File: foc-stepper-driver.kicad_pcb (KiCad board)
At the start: 4 copper layers, 42 x 42 mm, 72 parts, among them CN1 C42391660, CN2 C2839706, CN3 C2839705, CN4 C2839704, J2 TC2030, U1 DRV8962DDWR, U2 TYPE-C 16PLT-H10.0, U3 STM32G431CBT6, U6 AS5047P-ATSM, U7 TPS560430XDBVR, U8 SPX3819M5-L-3-3/TR, U9 TCAN3403DRQ1, X1 NX3215SA 32.768KHZ EXS00A-MU0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, X2 NDK NX2016SA-24MHZ-EXS00A-CS1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

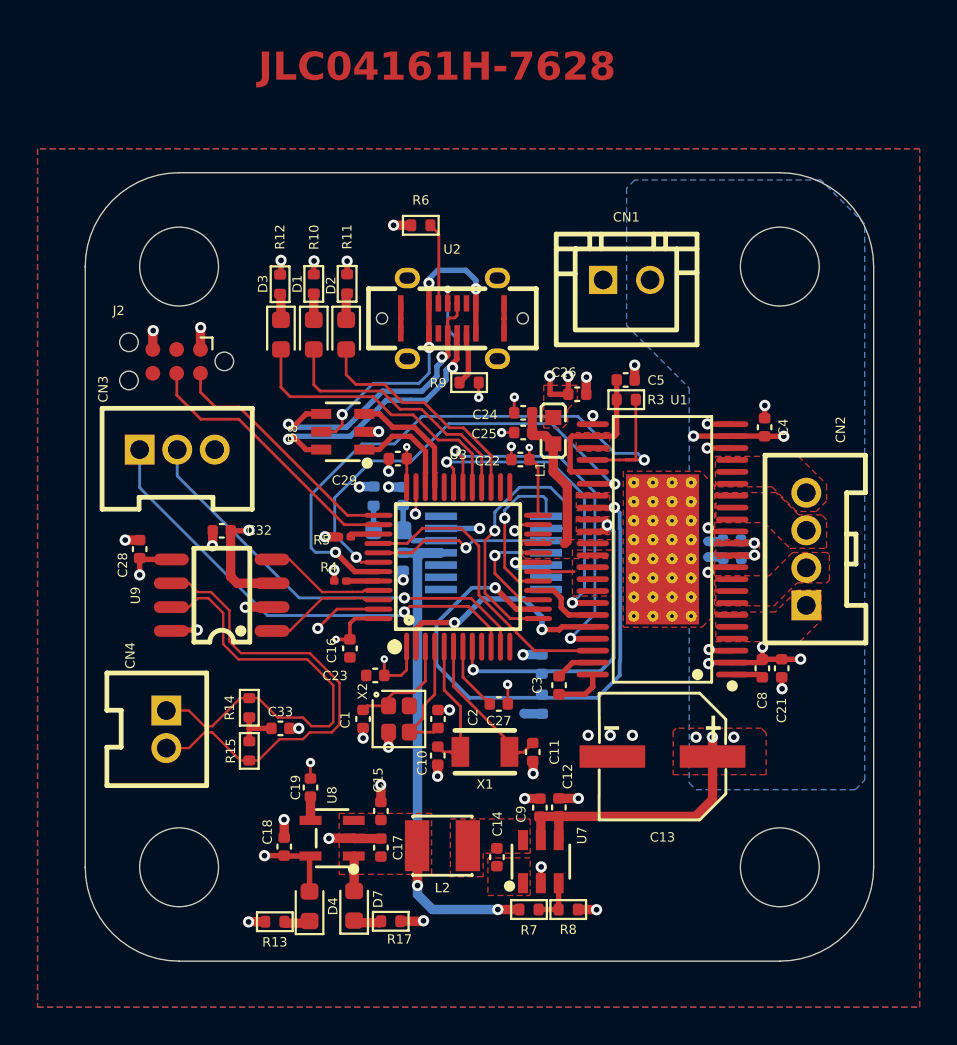
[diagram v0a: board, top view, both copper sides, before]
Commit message: update
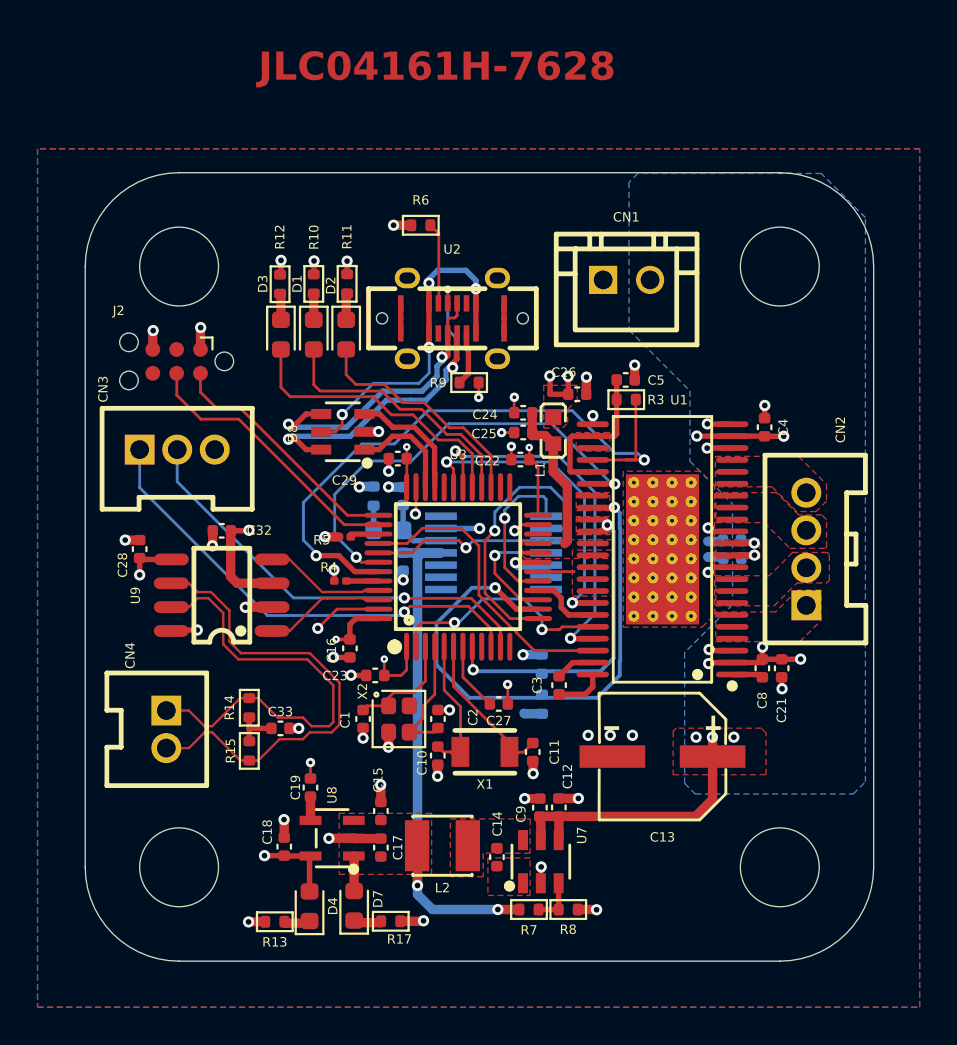
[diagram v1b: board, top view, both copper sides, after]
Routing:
- net GND: track 61.1 -> 62.8 mm, vias 54 -> 56
- net /DRV8962DDWR/DRV8962_nFAULT: track 33.9 -> 34.6 mm

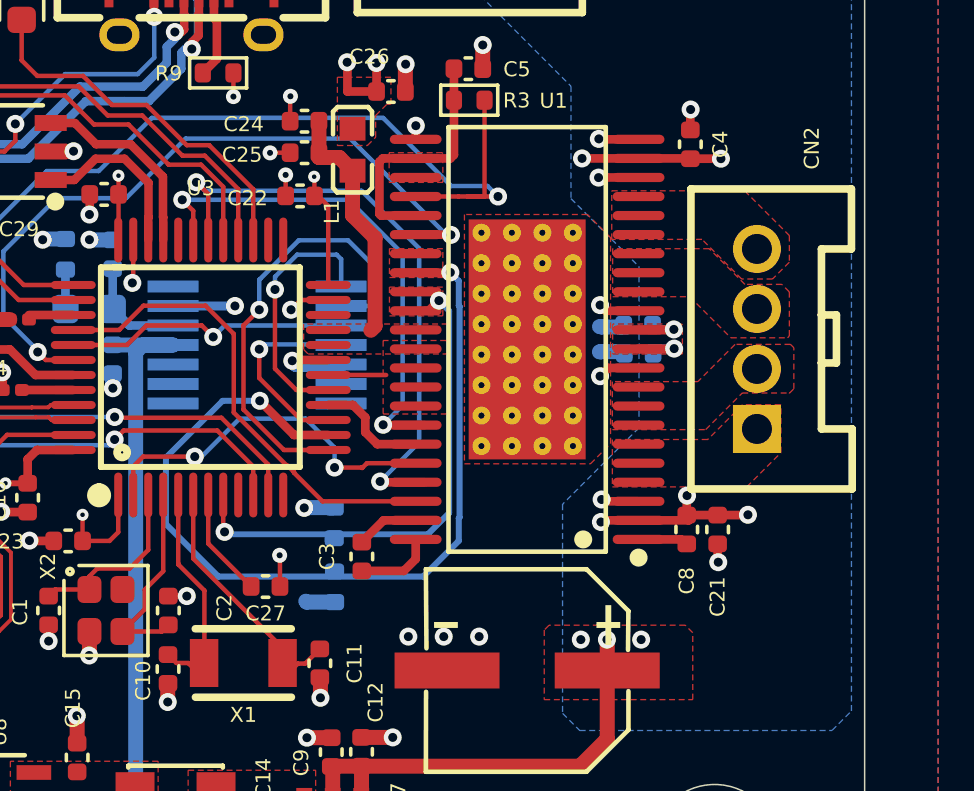
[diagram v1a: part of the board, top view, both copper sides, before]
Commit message: update
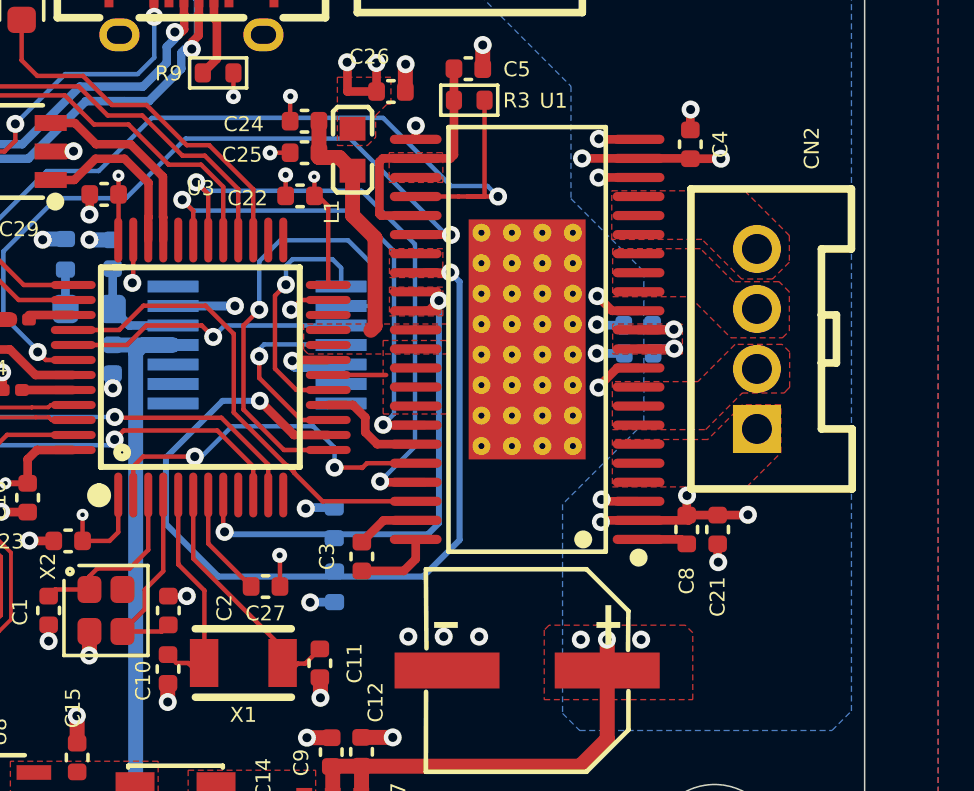
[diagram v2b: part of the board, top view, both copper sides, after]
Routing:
- net GND: track 62.8 -> 63.1 mm, vias 56 -> 59
